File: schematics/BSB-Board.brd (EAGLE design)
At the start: 29.7 x 53.3 mm, 23 parts, among them Q1 BC 547A, Q11 BC 557A, Q12 BC 547A, U1 4N25, U2 4N25

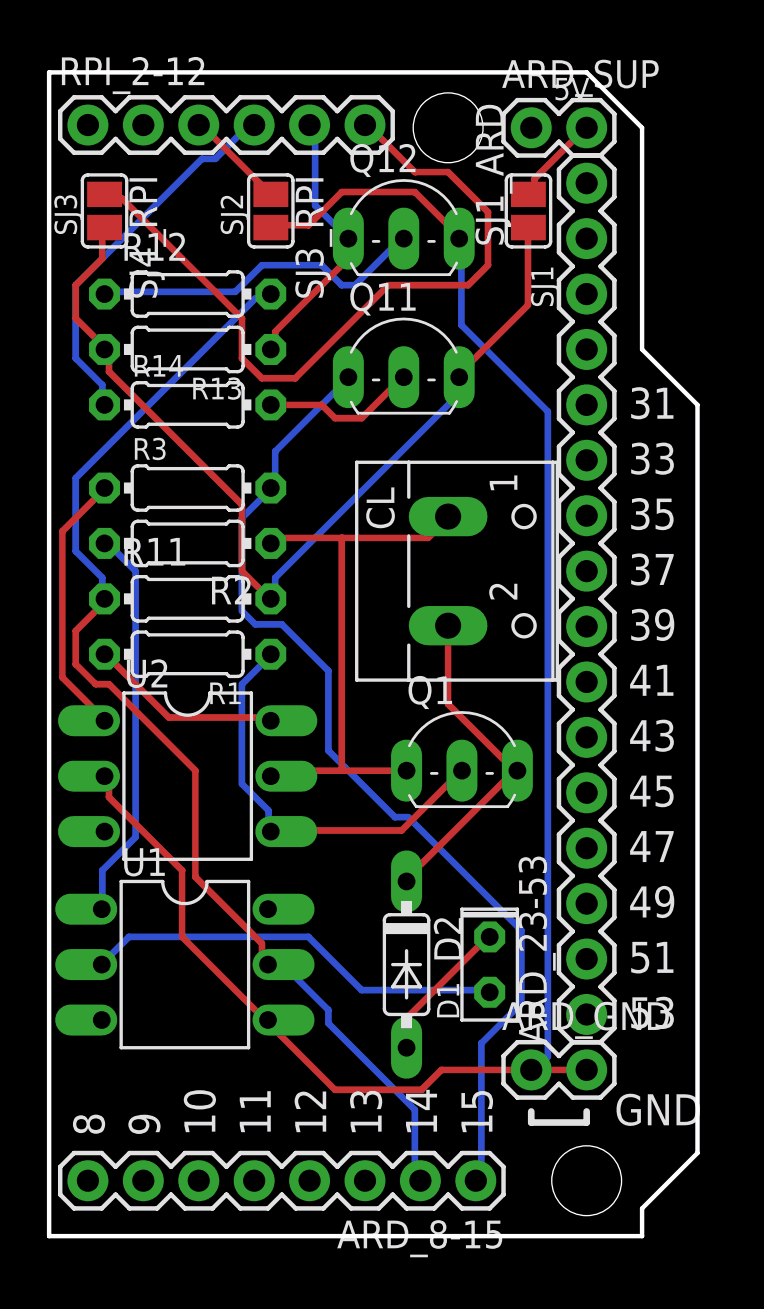
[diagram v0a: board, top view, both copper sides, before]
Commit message: Bugfixes
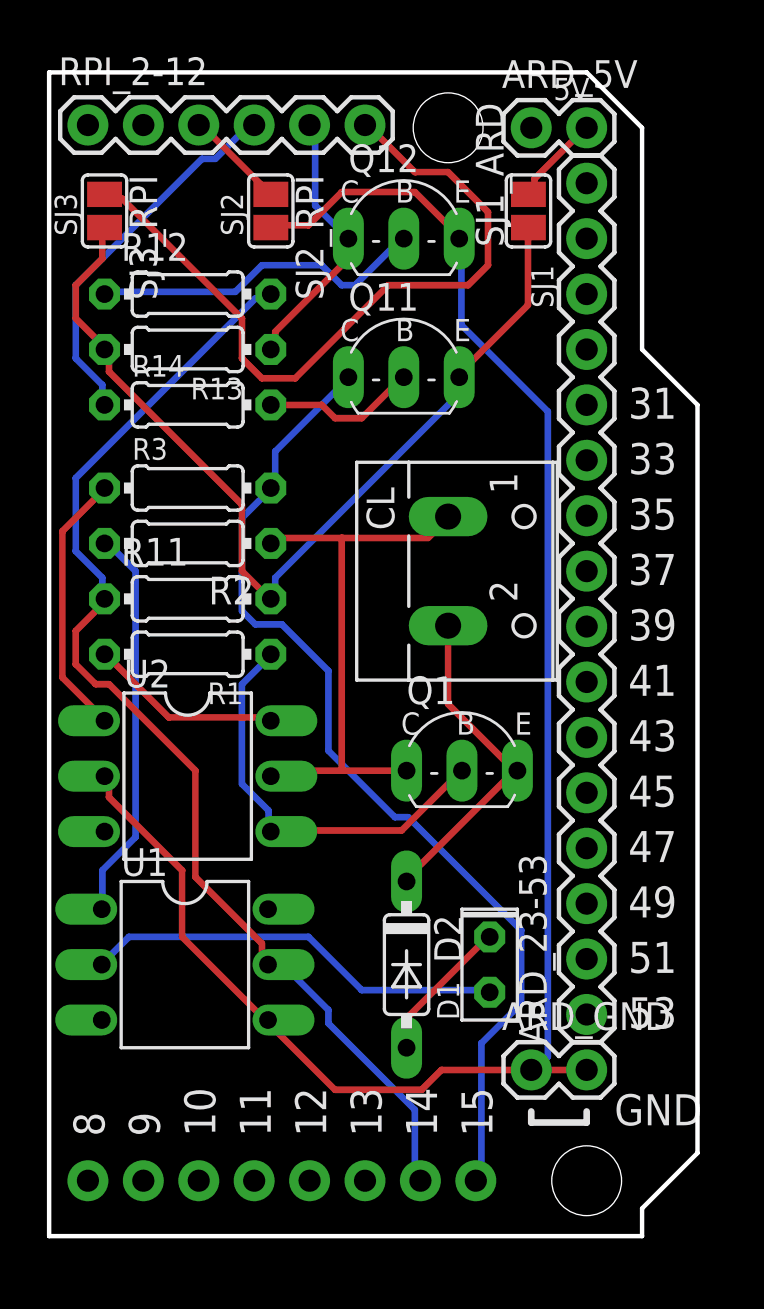
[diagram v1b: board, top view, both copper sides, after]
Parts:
- removed SJ4_RPI: Close for RPi, jumper:SJ
- added SJ2_RPI: Close for RPi, jumper:SJ
- moved ARD_8-15 17.8 mm to (1.78, 2.54), flipped to the bottom
- moved SJ3_RPI 7.62 mm to (2.54, 47.0)
- renumbered ARD_SUP to ARD_5V
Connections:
- net N$11 renamed ARD_PI_TXD
- net A14-RXD-ARD: now also ARD_8-15.7; no longer ARD_8-15.2
- net A15-TXD-ARD: now also ARD_8-15.8; no longer ARD_8-15.1
- net GND-ARD: now also SJ2_RPI.2; no longer SJ3_RPI.2
- net GPIO18-3V3-PI: now also SJ3_RPI.1; no longer SJ4_RPI.1
- net PIN6-GND-PI: now also SJ2_RPI.1; no longer SJ3_RPI.1
- net VCC: now also SJ3_RPI.2; no longer SJ4_RPI.2
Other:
- board text added: "B"
- board text added: "C"
- board text added: "E"
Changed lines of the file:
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@@
 <text x="13.843" y="32.385" size="1.016" layer="27" rot="R90">DB
 CL+</text>
+<text x="13.335" y="41.021" size="1.016" layer="21" font="vector" ratio="15">C</text>
+<text x="15.875" y="41.021" size="1.016" layer="21" font="vector" ratio="15">B</text>
+<text x="18.542" y="41.021" size="1.016" layer="21" font="vector" ratio="15">E</text>
+<text x="16.129" y="22.987" size="1.016" layer="21" font="vector" ratio="15">C</text>
+<text x="18.669" y="22.987" size="1.016" layer="21" font="vector" ratio="15">B</text>
+<text x="21.336" y="22.987" size="1.016" layer="21" font="vector" ratio="15">E</text>
+<text x="13.335" y="47.371" size="1.016" layer="21" font="vector" ratio="15">C</text>
+<text x="15.875" y="47.371" size="1.016" layer="21" font="vector" ratio="15">B</text>
+<text x="18.542" y="47.371" size="1.016" layer="21" font="vector" ratio="15">E</text>
 </plain>
 <attributes>
@@
 <elements>
 <element name="ARD_GND" library="SparkFun-Connectors" package="1X02" value="" x="22.098" y="7.62"/>
-<element name="ARD_SUP" library="SparkFun-Connectors" package="1X02" value="" x="22.098" y="50.8"/>
+<element name="ARD_5V" library="SparkFun-Connectors" package="1X02" value="" x="22.098" y="50.8"/>
 <element name="U1" library="optocoupler" package="DIL06" value="4N25" x="6.223" y="12.446" rot="R270">
 <attribute name="MF" value="" x="6.223" y="12.446" size="1.778" layer="27" rot="R270" display="off"/>
@@
 <attribute name="VALUE" x="12.446" y="36.068" size="1.27" layer="27" ratio="10"/>
 </element>
-<element name="SJ4_RPI" library="jumper" package="SJ" value="Close for RPi" x="2.54" y="46.99" rot="R270"/>
-<element name="SJ3_RPI" library="jumper" package="SJ" value="Close for RPi" x="10.16" y="46.99" rot="R270"/>
+<element name="SJ3_RPI" library="jumper" package="SJ" value="Close for RPi" x="2.54" y="46.99" rot="R270"/>
+<element name="SJ2_RPI" library="jumper" package="SJ" value="Close for RPi" x="10.16" y="46.99" rot="R270"/>
 <element name="SJ1_ARD" library="jumper" package="SJ" value="Close for Arduino" x="21.971" y="46.99" rot="R90"/>
 <element name="RPI_2-12" library="SparkFun-Connectors" package="1X06" value="" x="1.778" y="50.927">
@@
 </element>
 <element name="ARD_23-53" library="SparkFun-Connectors" package="1X16" value="" x="24.638" y="10.16" rot="R90"/>
-<element name="ARD_8-15" library="SparkFun-Connectors" package="1X08_ROUND" value="" x="19.558" y="2.54" rot="R180"/>
+<element name="ARD_8-15" library="SparkFun-Connectors" package="1X08_ROUND" value="" x="1.778" y="2.54" rot="MR180"/>
 </elements>
 <signals>
 <signal name="A14-RXD-ARD">
-<contactref element="R11" pad="1"/>
-<contactref element="R12" pad="2"/>
 <contactref element="U1" pad="5"/>
-<wire x1="2.4384" y1="30.1752" x2="2.4384" y2="29.2608" width="0.3048" layer="16"/>
-<wire x1="1.2192" y1="31.3944" x2="2.4384" y2="30.1752" width="0.3048" layer="16"/>
-<wire x1="1.2192" y1="34.7472" x2="1.2192" y2="31.3944" width="0.3048" layer="16"/>
-<wire x1="9.4488" y1="42.9768" x2="1.2192" y2="34.7472" width="0.3048" layer="16"/>
-<wire x1="10.0584" y1="42.9768" x2="9.4488" y2="42.9768" width="0.3048" layer="16"/>
-<wire x1="2.4384" y1="29.2608" x2="2.54" y2="29.21" width="0.3048" layer="16"/>
-<wire x1="10.0584" y1="42.9768" x2="10.16" y2="43.18" width="0.3048" layer="16"/>
 <wire x1="9.7536" y1="13.4112" x2="9.7536" y2="12.4968" width="0.3048" layer="1"/>
 <wire x1="6.7056" y1="16.4592" x2="9.7536" y2="13.4112" width="0.3048" layer="1"/>
@@
 <wire x1="2.4384" y1="28.956" x2="1.2192" y2="27.7368" width="0.3048" layer="1"/>
 <wire x1="9.7536" y1="12.4968" x2="10.033" y2="12.446" width="0.3048" layer="1"/>
-<wire x1="2.4384" y1="28.956" x2="2.54" y2="29.21" width="0.3048" layer="1"/>
-<contactref element="ARD_8-15" pad="2"/>
+<contactref element="R11" pad="1"/>
+<contactref element="R12" pad="2"/>
+<contactref element="ARD_8-15" pad="7"/>
+<wire x1="2.4384" y1="30.1752" x2="2.4384" y2="29.2608" width="0.3048" layer="16"/>
+<wire x1="1.2192" y1="31.3944" x2="2.4384" y2="30.1752" width="0.3048" layer="16"/>
+<wire x1="1.2192" y1="34.7472" x2="1.2192" y2="31.3944" width="0.3048" layer="16"/>
+<wire x1="9.4488" y1="42.9768" x2="1.2192" y2="34.7472" width="0.3048" layer="16"/>
+<wire x1="10.0584" y1="42.9768" x2="9.4488" y2="42.9768" width="0.3048" layer="16"/>
+<wire x1="2.4384" y1="29.2608" x2="2.54" y2="29.21" width="0.3048" layer="16"/>
+<wire x1="10.0584" y1="42.9768" x2="10.16" y2="43.18" width="0.3048" layer="16"/>
 <wire x1="16.764" y1="5.7912" x2="16.764" y2="2.7432" width="0.3048" layer="16"/>
 <wire x1="12.8016" y1="9.7536" x2="16.764" y2="5.7912" width="0.3048" layer="16"/>
@@
 <wire x1="16.764" y1="2.7432" x2="17.018" y2="2.54" width="0.3048" layer="16"/>
 <wire x1="10.0584" y1="12.192" x2="10.033" y2="12.446" width="0.3048" layer="16"/>
+<wire x1="2.4384" y1="28.956" x2="2.54" y2="29.21" width="0.3048" layer="1"/>
 </signal>
 <signal name="A15-TXD-ARD">
@@
 <wire x1="10.3632" y1="34.4424" x2="10.16" y2="34.29" width="0.3048" layer="16"/>
 <wire x1="13.716" y1="39.3192" x2="13.716" y2="39.37" width="0.3048" layer="16"/>
-<contactref element="ARD_8-15" pad="1"/>
+<contactref element="ARD_8-15" pad="8"/>
 <wire x1="19.812" y1="8.8392" x2="19.812" y2="2.7432" width="0.3048" layer="16"/>
 <wire x1="21.6408" y1="10.668" x2="19.812" y2="8.8392" width="0.3048" layer="16"/>
@@
 <wire x1="21.336" y1="21.336" x2="21.463" y2="21.336" width="0.3048" layer="1"/>
 </signal>
-<signal name="N$11">
+<signal name="ARD_PI_TXD">
 <contactref element="U2" pad="1"/>
 <contactref element="R3" pad="1"/>
@@
 <contactref element="Q11" pad="E"/>
 <contactref element="R11" pad="2"/>
-<contactref element="SJ4_RPI" pad="2"/>
+<contactref element="SJ3_RPI" pad="2"/>
 <contactref element="SJ1_ARD" pad="1"/>
 <wire x1="2.4384" y1="44.8056" x2="2.4384" y2="46.0248" width="0.3048" layer="1"/>
@@
 <contactref element="U1" pad="4"/>
 <contactref element="Q12" pad="E"/>
-<contactref element="SJ3_RPI" pad="2"/>
+<contactref element="SJ2_RPI" pad="2"/>
 <wire x1="2.7432" y1="20.1168" x2="2.7432" y2="21.0312" width="0.3048" layer="1"/>
 <wire x1="6.096" y1="16.764" x2="2.7432" y2="20.1168" width="0.3048" layer="1"/>
@@
 </signal>
 <signal name="GPIO18-3V3-PI">
-<contactref element="SJ4_RPI" pad="1"/>
+<contactref element="SJ3_RPI" pad="1"/>
 <contactref element="RPI_2-12" pad="6"/>
 <wire x1="3.3528" y1="47.5488" x2="2.7432" y2="47.5488" width="0.3048" layer="1"/>
@@
 </signal>
 <signal name="PIN6-GND-PI">
-<contactref element="SJ3_RPI" pad="1"/>
+<contactref element="SJ2_RPI" pad="1"/>
 <contactref element="RPI_2-12" pad="3"/>
 <wire x1="7.0104" y1="50.9016" x2="10.16" y2="47.752" width="0.3048" layer="1"/>
@@
 </signal>
 <signal name="5V-ARD">
-<contactref element="ARD_SUP" pad="2"/>
+<contactref element="ARD_5V" pad="2"/>
 <contactref element="SJ1_ARD" pad="2"/>
 <wire x1="22.2504" y1="48.4632" x2="22.2504" y2="47.8536" width="0.3048" layer="1"/>
